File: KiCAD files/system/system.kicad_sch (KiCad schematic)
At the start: 14 parts, among them J1 Input, J2 Conn_01x04_Female, SW1 SW_Push, U1 ATmega328P-P, Y1 Crystal

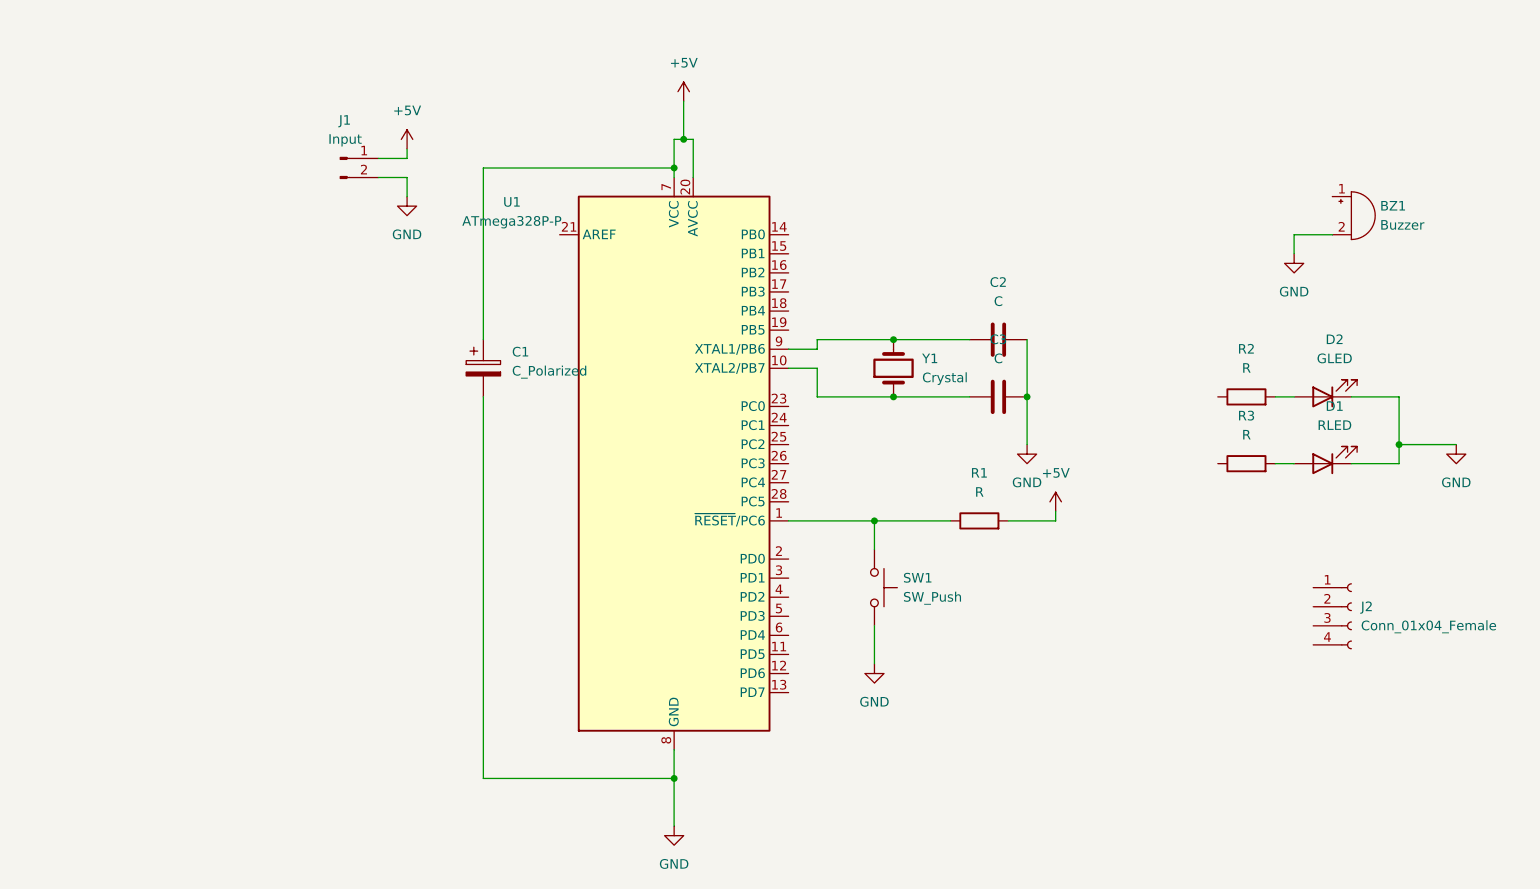
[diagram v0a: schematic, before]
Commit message: Update schematics of system
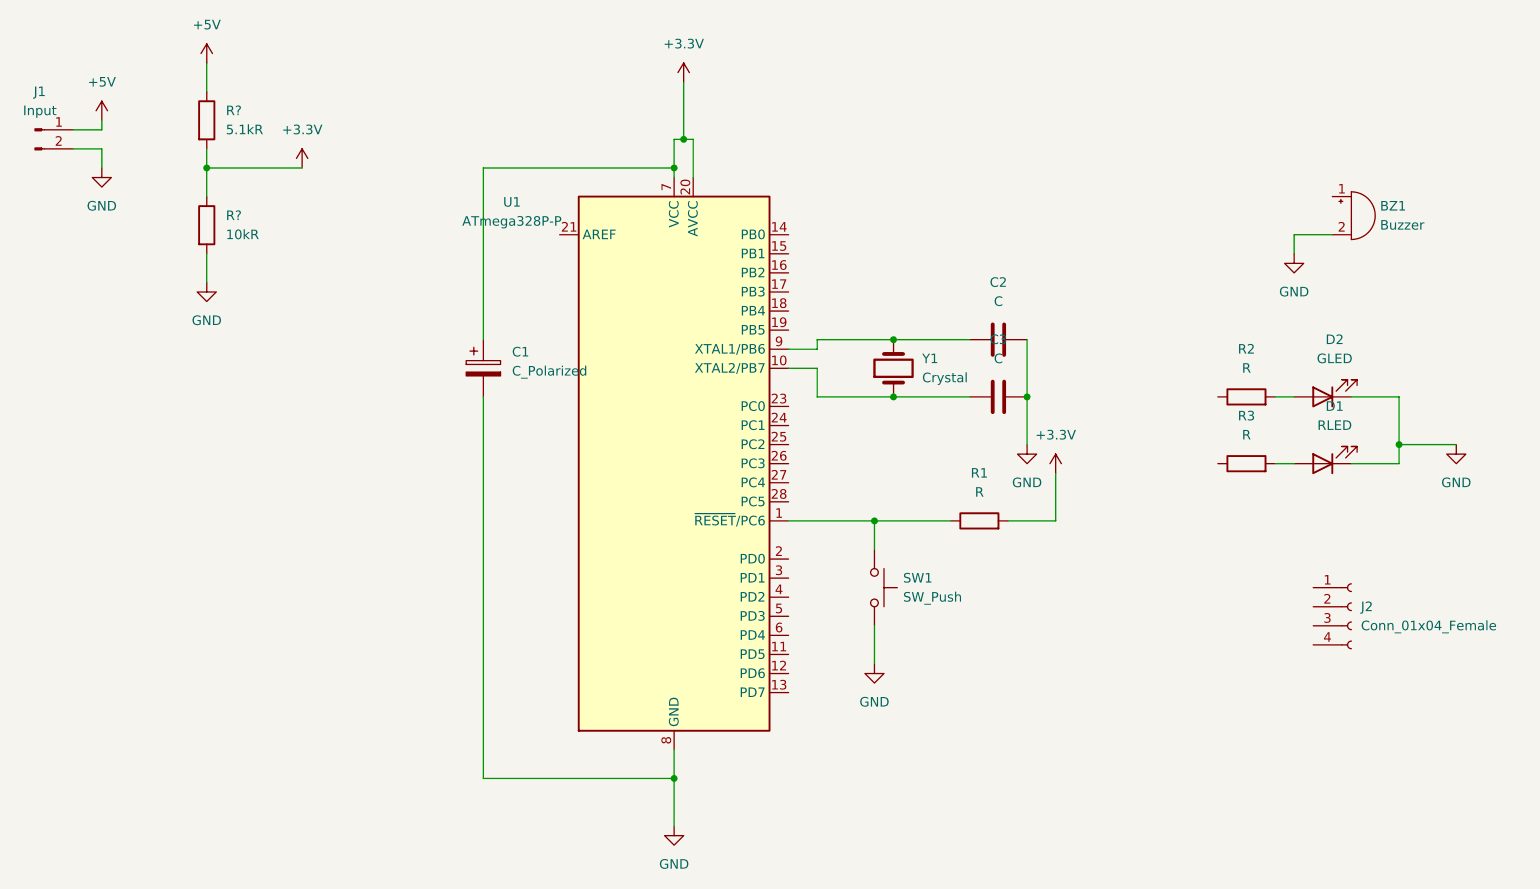
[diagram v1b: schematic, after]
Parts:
- added R?: 10kR, Resistor_THT:R_Axial_DIN0207_L6.3mm_D2.5mm_P10.16mm_Horizontal, symbol Device:R
- added R?: 5.1kR, Resistor_THT:R_Axial_DIN0207_L6.3mm_D2.5mm_P10.16mm_Horizontal, symbol Device:R
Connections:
- net +5V: now also R?.1; no longer C1.1, R1.2, U1.20 (AVCC), U1.7 (VCC)
- net GND: now also R?.2
- new net +3.3V: C1.1, R1.2, R?.1, R?.2, U1.20 (AVCC), U1.7 (VCC)
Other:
- moved on the sheet: J1
